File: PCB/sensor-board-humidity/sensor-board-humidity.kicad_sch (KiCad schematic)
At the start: 10 parts, among them U1 MAGNETIC POGO CONN., U2 MAGNETIC POGO CONN.

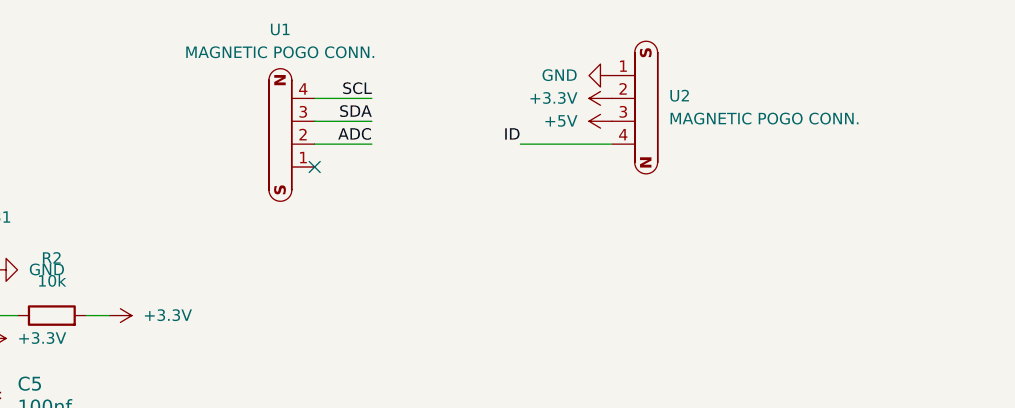
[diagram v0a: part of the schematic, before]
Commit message: made some changes
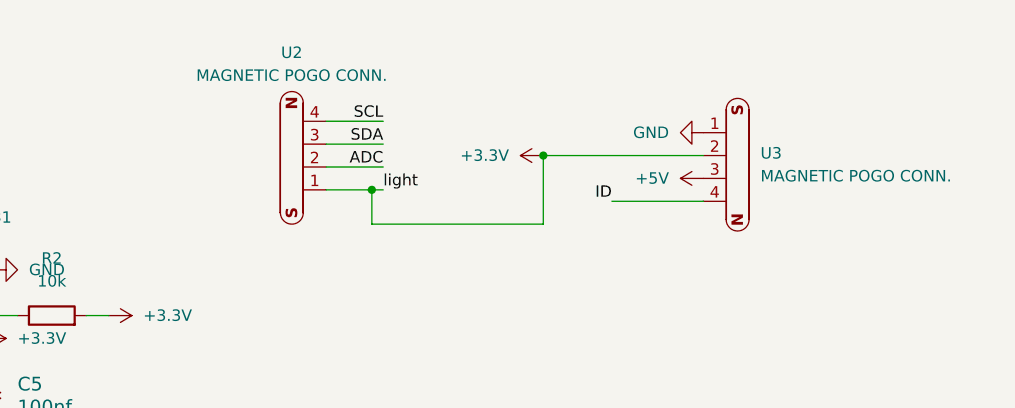
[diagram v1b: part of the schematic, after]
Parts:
- removed U1: MAGNETIC POGO CONN., batteryholder:MAGNETIC POGO CONN., symbol magnetic_pogo_conn.:MAGNETIC_POGO_CONN.
- added U2: MAGNETIC POGO CONN., batteryholder:MAGNETIC POGO CONN., symbol magnetic_pogo_conn.:MAGNETIC_POGO_CONN.
- renumbered U2 to U3
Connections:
- net +3.3V: now also U2.1
- net ADC: now also U2.2
- net SCL: now also U2.4
- net SDA: now also U2.3
- no-connect marks 2 -> 1
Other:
- moved on the sheet: U3
